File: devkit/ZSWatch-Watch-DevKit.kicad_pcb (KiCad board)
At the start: 4 copper layers, 100 x 70 mm, 129 parts, among them IC401 nPM1300-QEXX, IC501 APDS-9306-065, IC502 BMI270, IC503 LIS2MDLTR, IC504 BMP581, IC505 DRV2603RUNT, IC506 PCA9306JK, IC507 RV-8263-C8, IC601 FAN5622SX, IC602 USBLC6-2P6, IC603 MX25U51245GZ4I00, IC604 NTS0104GU12, M601 NORA-B106, Q401 PMZ550UNEYL, Q402 PMZ550UNEYL, Q403 PMZ550UNEYL, Q404 PMZB320UPEYL, X401 Battery, X402 Battery, X403 Power, X501 Current, X502 I2S, X503 Current, X504 I2C, X505 Current, X506 Current, X507 Current, X508 Current, X509 Motor, X510 Current, X601 DEBUG, X602 Current, X603 Device, X604 UART, X605 GPIO, X606 Current, X607 IO Current, X608 Display, X609 Touch Current, X610 LED Current

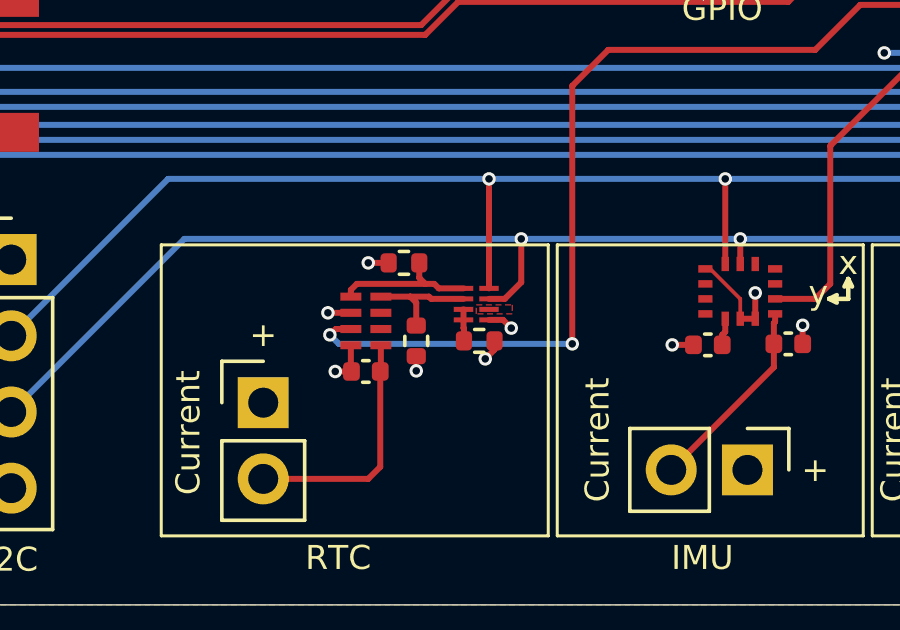
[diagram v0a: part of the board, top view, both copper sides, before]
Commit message: Revert "Bug: Issue #172"
This reverts commit d2b21792fba04b32ee89f1631bab4de80096e44a.
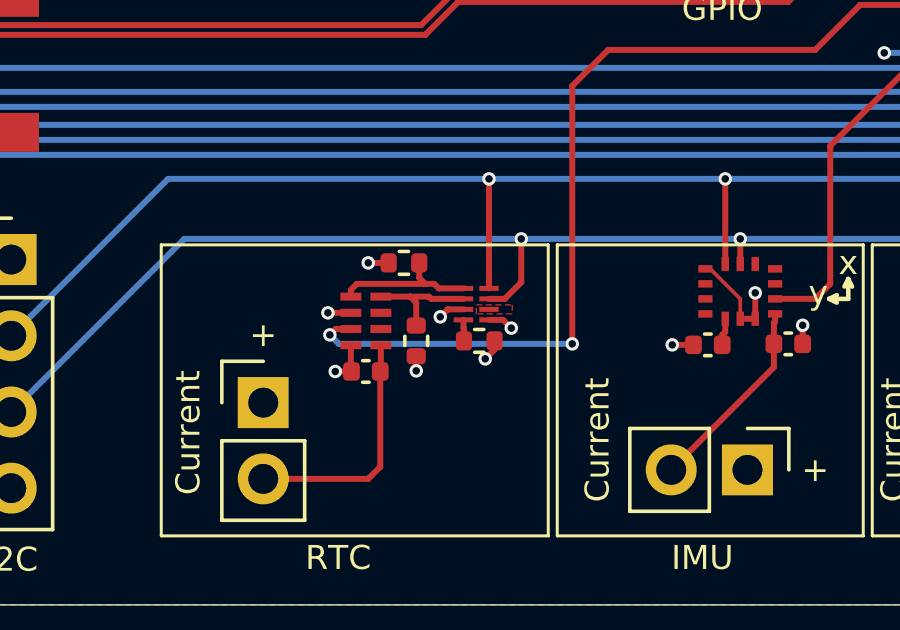
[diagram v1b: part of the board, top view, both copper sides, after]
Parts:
- R503: value 200k -> 100k
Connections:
- IC506 pad 7: Net-(IC506-EN) -> /Project Architecture/Peripherals/VBAT
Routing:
- net /Project Architecture/Peripherals/VBAT: track 22.1 -> 23.0 mm, vias 5 -> 6
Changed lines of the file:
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@@
 			(size 0.65 0.17)
 			(layers "F.Cu" "F.Mask" "F.Paste")
-			(net 147 "Net-(IC506-EN)")
+			(net 5 "/Project Architecture/Peripherals/VBAT")
 			(pinfunction "VCC_{2}")
 			(pintype "power_in")
@@
 			)
 		)
-		(property "Value" "200k"
+		(property "Value" "100k"
 			(at 0 1.17 0)
 			(layer "F.Fab")
@@
 			)
 		)
-		(property "manf#" "RC0402FR-07200KL"
+		(property "manf#" "RC0402FR-07100KL"
 			(at 0 0 0)
 			(unlocked yes)
@@
 			)
 		)
-		(property "mouser#" "603-RC0402FR-07200KL"
+		(property "mouser#" "603-RC0402FR-07100KL"
 			(at 0 0 0)
 			(unlocked yes)
@@
 	)
 	(segment
+		(start 209.875 174.15)
+		(end 209.35 174.15)
+		(width 0.2)
+		(layer "F.Cu")
+		(net 5)
+	)
+	(segment
 		(start 227.8 117.5)
 		(end 226.8 116.5)
@@
 	)
 	(segment
+		(start 209.35 174.15)
+		(end 209.1 174.4)
+		(width 0.2)
+		(layer "F.Cu")
+		(net 5)
+	)
+	(segment
 		(start 203.87 177.23)
 		(end 203.9 177.2)
@@
 	)
 	(via
+		(at 209.1 174.4)
+		(size 0.45)
+		(drill 0.25)
+		(layers "F.Cu" "B.Cu")
+		(net 5)
+	)
+	(via
 		(at 228.4 119.8)
 		(size 0.45)
@@
 		(end 209.875 174.5)
 		(width 0.2)
-		(layer "F.Cu")
-		(net 147)
-	)
-	(segment
-		(start 209.875 174.15)
-		(end 209.875 174.5)
-		(width 0.2)
